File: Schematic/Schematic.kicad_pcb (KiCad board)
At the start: 2 copper layers, 53.3 x 45.7 mm, 6 parts, among them J1 S2B-PH-K-S_LF__SN_, P1 282837-2, P2 282837-2, U1 NRF52840-DONGLE, U2 L293D

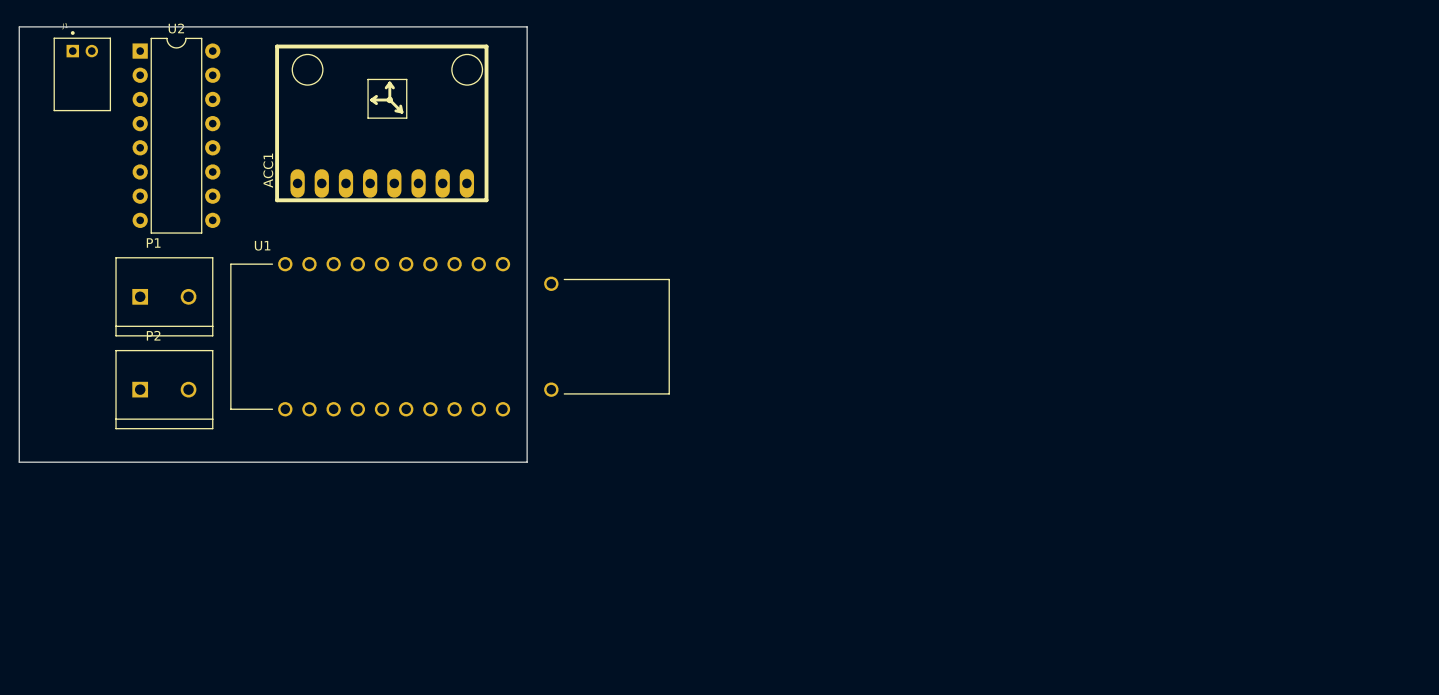
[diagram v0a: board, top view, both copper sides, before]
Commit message: PCB: Added all neecesseary symbols, footprints and 3d models
-create an demo PCB
-create 3dvis folder with apperance of the boards
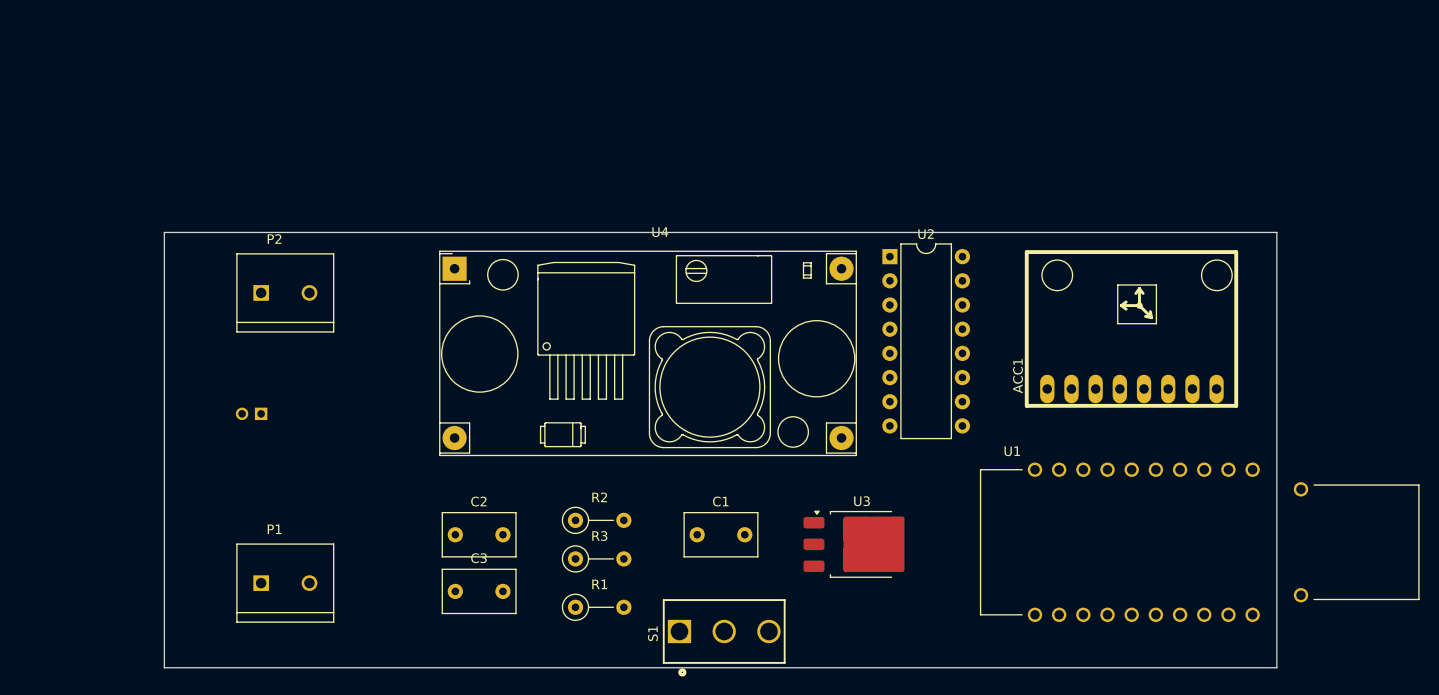
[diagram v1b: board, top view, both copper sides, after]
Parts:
- added C1: 100uF, Capacitor_THT:C_Disc_D7.5mm_W4.4mm_P5.00mm, F.Cu at (175.3, 116.8)
- added C2: 100uF, Capacitor_THT:C_Disc_D7.5mm_W4.4mm_P5.00mm, F.Cu at (149.9, 116.8)
- added C3: 100uF, Capacitor_THT:C_Disc_D7.5mm_W4.4mm_P5.00mm, F.Cu at (149.9, 122.8)
- added R1: 100R, Resistor_THT:R_Axial_DIN0207_L6.3mm_D2.5mm_P5.08mm_Vertical, F.Cu at (162.6, 124.5)
- added R2: 100R, Resistor_THT:R_Axial_DIN0207_L6.3mm_D2.5mm_P5.08mm_Vertical, F.Cu at (162.6, 115.3)
- added R3: 100R, Resistor_THT:R_Axial_DIN0207_L6.3mm_D2.5mm_P5.08mm_Vertical, F.Cu at (162.6, 119.4)
- added S1: 1101M2S3CQE2, 1101M2S3CQE2:SW_1101M2S3CQE2, F.Cu at (178.2, 127.0)
- added U3: LM1117DT-3.3, Package_TO_SOT_SMD:TO-252-3_TabPin2, F.Cu at (192.6, 117.9)
- added U4: YAAJ_DCDC_StepDown_LM2596, lm256:YAAJ_DCDC_StepDown_LM2596, F.Cu at (149.9, 88.9)
- J1: moved to B.Cu
- moved ACC1 81.6 mm to (232.0, 103.3)
- moved U1 81.6 mm to (228.1, 117.6)
- moved U2 81.6 mm to (195.6, 87.6)
- moved J1 42.0 mm to (128.5, 104.1), turned to 180 degrees
- moved P1 32.6 mm to (132.1, 121.9)
- moved P2 16.3 mm to (132.1, 91.4)
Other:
- board size 53.3 x 45.7 mm -> 116.8 x 45.7 mm
